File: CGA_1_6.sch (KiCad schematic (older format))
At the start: 10 parts, among them U50 2118, U51 2118, U52 2118, U53 2118, U54 2118, U55 2118, U56 2118, U57 2118, U60 74LS374, U61 74LS374

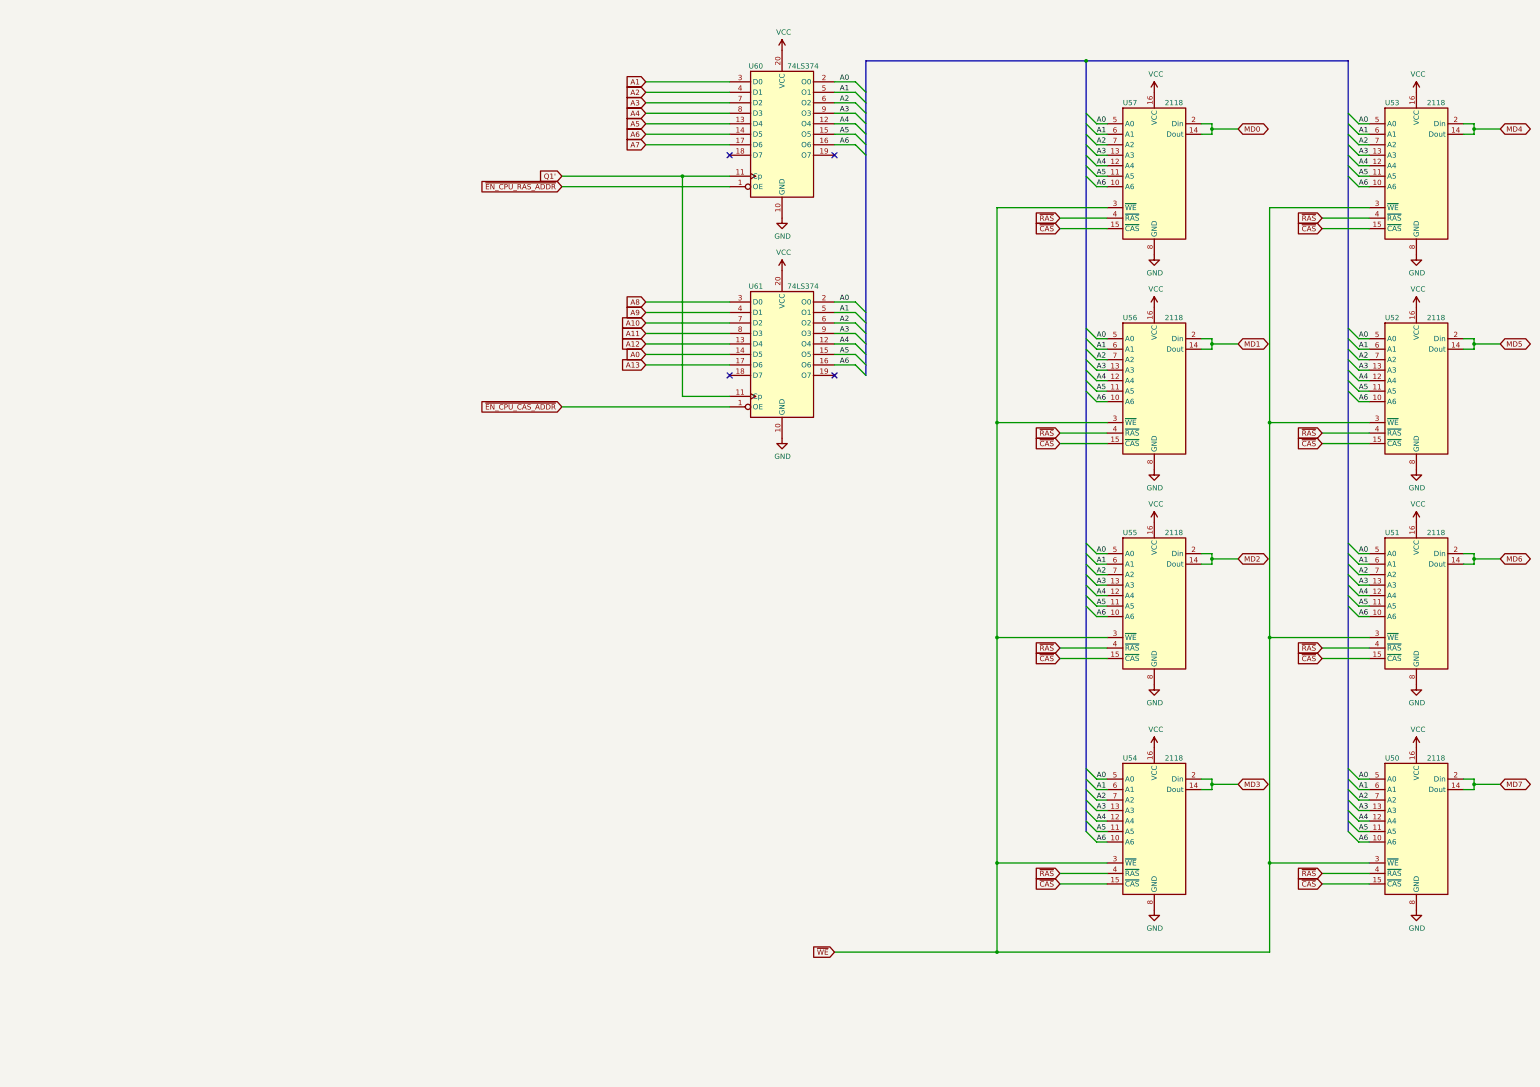
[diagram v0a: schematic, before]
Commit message: Complete a sheet
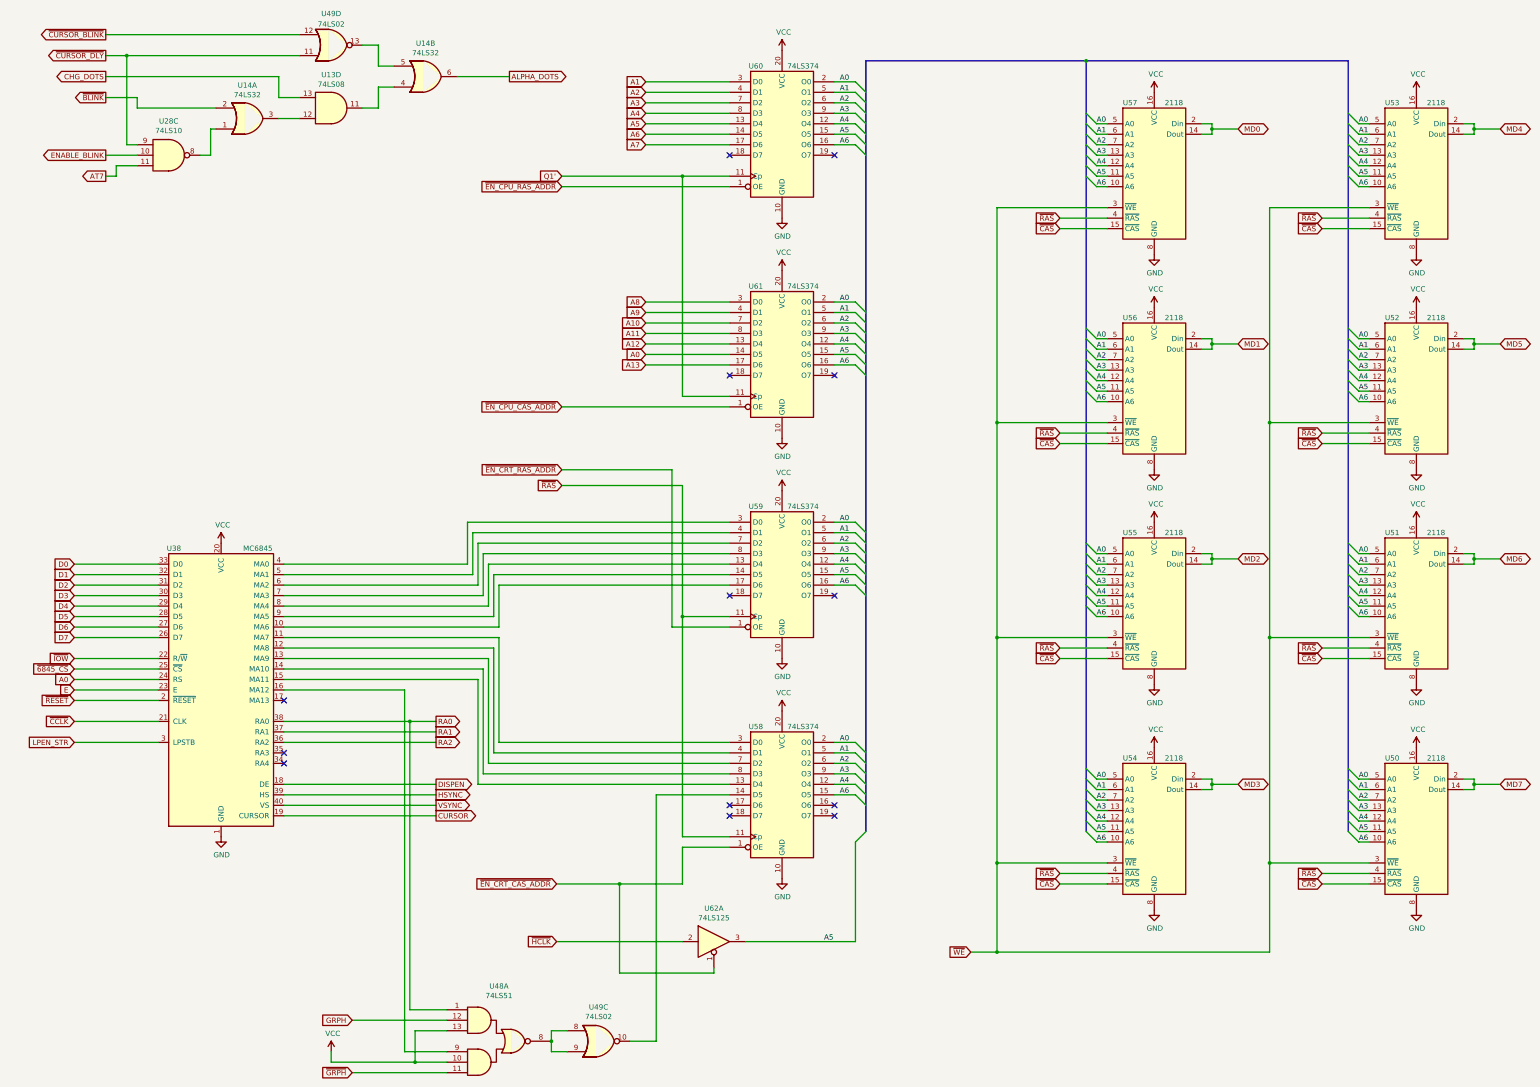
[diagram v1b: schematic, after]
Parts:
- added U13: 74LS08, Package_DIP:DIP-14_W7.62mm_LongPads, symbol 74xx:74LS08
- added U14: 74LS32, Package_DIP:DIP-14_W7.62mm_LongPads, symbol 74xx:74LS32
- added U28: 74LS10, Package_DIP:DIP-14_W7.62mm_LongPads, symbol 74xx:74LS10
- added U38: MC6845, Package_DIP:DIP-40_W15.24mm_LongPads, symbol GPU:MC6845
- added U48: 74LS51, Package_DIP:DIP-14_W7.62mm_LongPads, symbol 74xx:74LS51
- added U49: 74LS02, symbol 74xx:74LS02
- added U58, U59: 74LS374, Package_DIP:DIP-20_W7.62mm_LongPads, symbol 74xx:74LS374
- added U62: 74LS125, Package_DIP:DIP-14_W10.16mm_LongPads, symbol 74xx:74LS125
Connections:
- net A0: now also U38.24 (RS), U58.2 (O0), U59.2 (O0)
- net A1: now also U58.5 (O1), U59.5 (O1)
- net A2: now also U58.6 (O2), U59.6 (O2)
- net A3: now also U58.9 (O3), U59.9 (O3)
- net A4: now also U58.12 (O4), U59.12 (O4)
- net A5: now also U59.15 (O5), U62.3
- net A6: now also U58.15 (O5), U59.16 (O6)
- net GND: now also U38.1 (GND), U58.10 (GND), U59.10 (GND)
- net VCC: now also U38.20 (VCC), U48.10, U48.13, U58.20 (VCC), U59.20 (VCC)
- net ~RAS: now also U58.11 (Cp), U59.11 (Cp)
- new net: U14.5, U49.13
- new net: U13.11, U14.4
- new net: U13.12, U14.3
- new net: U14.1, U28.8
- new net: U38.8 (MA4), U59.13 (D4)
- new net: U38.9 (MA5), U59.14 (D5)
- new net: U38.10 (MA6), U59.17 (D6)
- new net: U38.4 (MA0), U59.3 (D0)
- new net: U38.5 (MA1), U59.4 (D1)
- new net: U38.6 (MA2), U59.7 (D2)
- new net: U38.7 (MA3), U59.8 (D3)
- new net: U38.15 (MA11), U58.13 (D4)
- new net: U49.10, U58.14 (D5)
- new net: U38.11 (MA7), U58.3 (D0)
- new net: U38.12 (MA8), U58.4 (D1)
- new net: U38.13 (MA9), U58.7 (D2)
- new net: U38.14 (MA10), U58.8 (D3)
- new net: U48.8, U49.8, U49.9
- new net: U38.16 (MA12), U48.9
- new net ALPHA_DOTS: U14.6
- new net AT7: U28.11
- new net CHG_DOTS: U13.13
- new net CURSOR: U38.19 (CURSOR)
- new net D0: U38.33 (D0)
- new net D1: U38.32 (D1)
- new net D2: U38.31 (D2)
- new net D3: U38.30 (D3)
- new net D4: U38.29 (D4)
- new net D5: U38.28 (D5)
- new net D6: U38.27 (D6)
- new net D7: U38.26 (D7)
- new net DISPEN: U38.18 (DE)
- new net E: U38.23 (E)
- new net ENABLE_BLINK: U28.10
- new net GRPH: U48.12
- new net HSYNC: U38.39 (HS)
- new net LPEN_STR: U38.3 (LPSTB)
- new net RA0: U38.38 (RA0), U48.1
- new net RA1: U38.37 (RA1)
- new net RA2: U38.36 (RA2)
- new net VSYNC: U38.40 (VS)
- new net ~6845_CS: U38.25 (~CS)
- new net ~BLINK: U14.2
- new net ~CCLK: U38.21 (CLK)
- new net ~CURSOR_BLINK: U49.12
- new net ~CURSOR_DLY: U28.9, U49.11
- new net ~EN_CRT_CAS_ADDR: U58.1 (OE), U62.1
- new net ~EN_CRT_RAS_ADDR: U59.1 (OE)
- new net ~GRPH: U48.11
- new net ~HCLK: U62.2
- new net ~IOW: U38.22 (R/~W)
- new net ~RESET: U38.2 (~RESET)
- no-connect marks 4 -> 13
